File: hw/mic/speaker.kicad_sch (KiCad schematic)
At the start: 4 parts, among them U6 MAX98357A

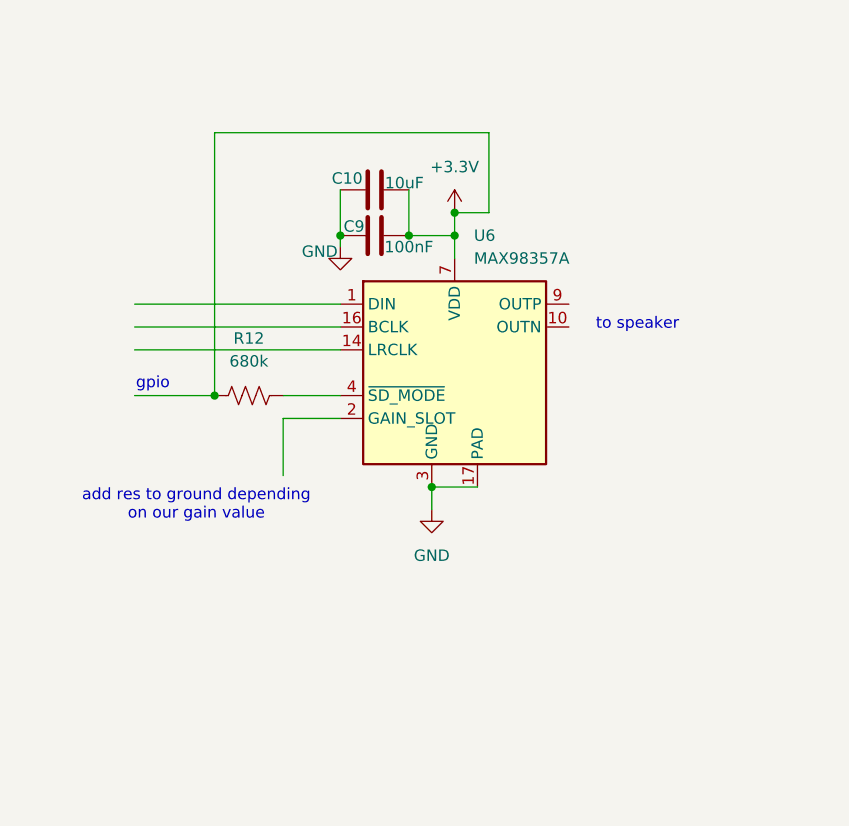
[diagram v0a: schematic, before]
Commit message: updated schema with speaker addition
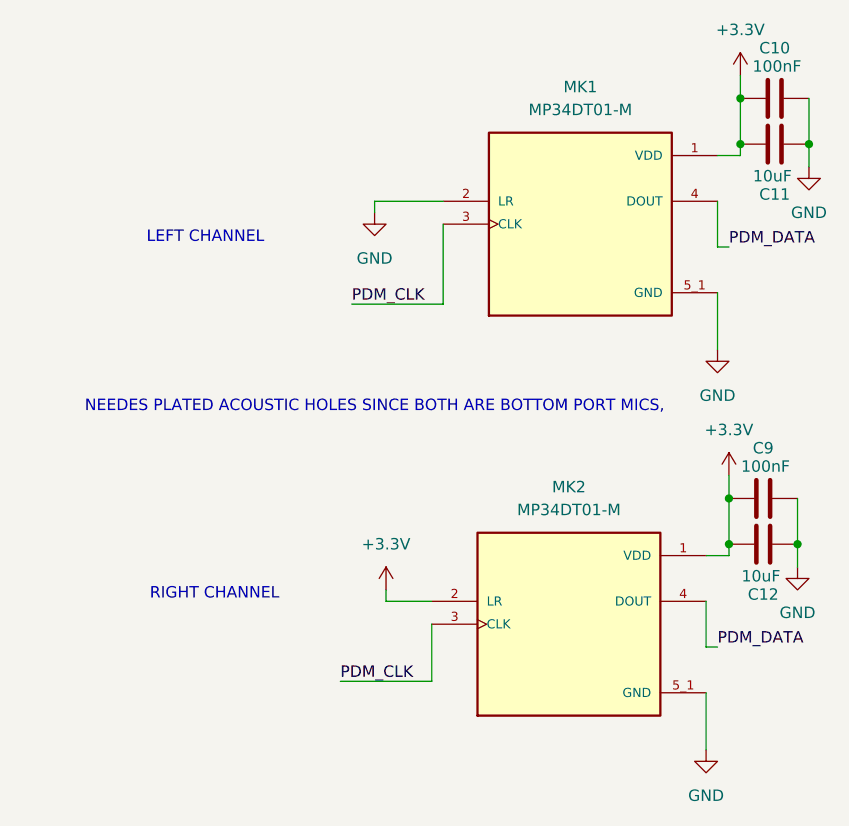
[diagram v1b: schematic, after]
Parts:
- removed R12: 680k, symbol Device:R_US
- removed U6: MAX98357A, Package_DFN_QFN:TQFN-16-1EP_3x3mm_P0.5mm_EP1.23x1.23mm, symbol Audio:MAX98357A
- added C11, C12: 10uF, symbol Device:C
- added MK1, MK2: MP34DT01-M, MP34DT01-M:MIC_MP34DT01-M, symbol MP34DT01-M:MP34DT01-M
- C10: value 10uF -> 100nF
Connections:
- net +3.3V: now also C11.2, C12.2, MK1.1 (VDD), MK2.1 (VDD), MK2.2 (LR)
- net GND: now also C11.1, C12.1, MK1.2 (LR), MK1.5_1 (GND), MK1.5_2 (GND), MK1.5_3 (GND), MK1.5_4 (GND), MK2.5_1 (GND), MK2.5_2 (GND), MK2.5_3 (GND), MK2.5_4 (GND)
- new net PDM_CLK: MK1.3 (CLK), MK2.3 (CLK)
- new net PDM_DATA: MK1.4 (DOUT), MK2.4 (DOUT)
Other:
- note added: "LEFT CHANNEL"
- note added: "NEEDES PLATED ACOUSTIC HOLES SINCE BOTH ARE BOTTOM PORT MICS,"
- note added: "RIGHT CHANNEL"
- note removed: "add res to ground depending on our gain value"
- note removed: "gpio"
- note removed: "to speaker"
